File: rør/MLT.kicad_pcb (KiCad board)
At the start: 2 copper layers, 69 x 128.5 mm, 44 parts, among them J1 PJ301M-12, J10 PJ301M-12, J11 PJ301M-12, J12 PJ301M-12, J2 PJ301M-12, J3 PJ301M-12, J4 PJ301M-12, J5 PJ301M-12, J6 PJ301M-12, J7 PJ301M-12, J8 PJ301M-12, J9 PJ301M-12, U1 TL074, U2 TL074, U3 TL074

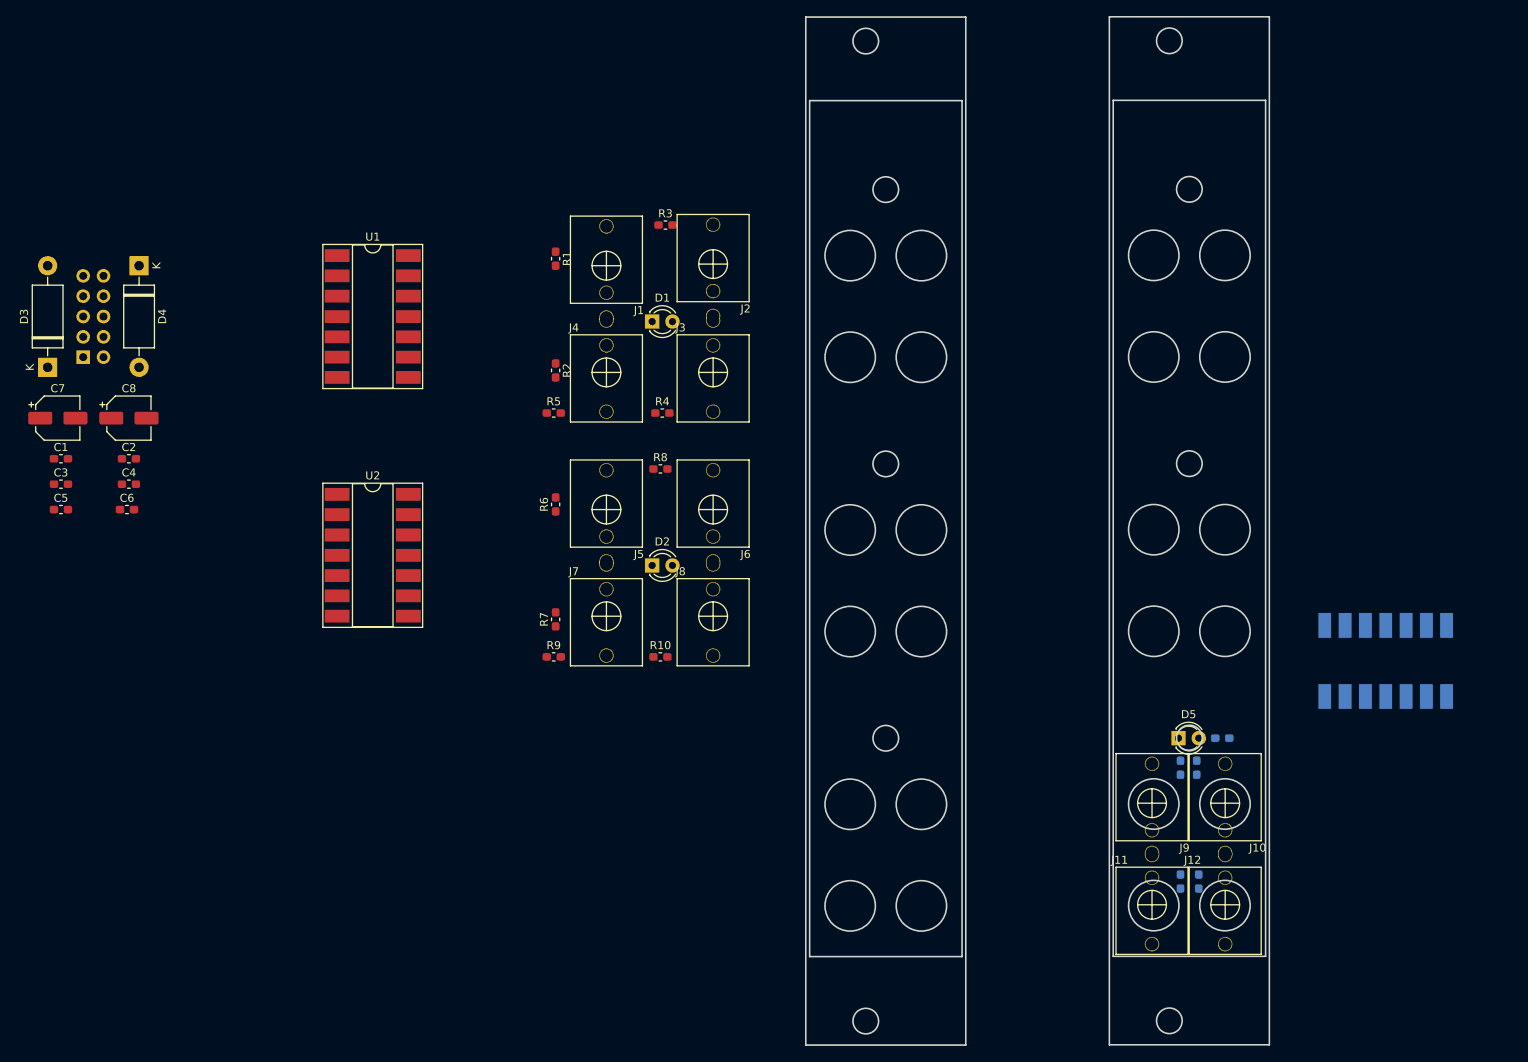
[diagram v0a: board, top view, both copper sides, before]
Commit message: mlt update
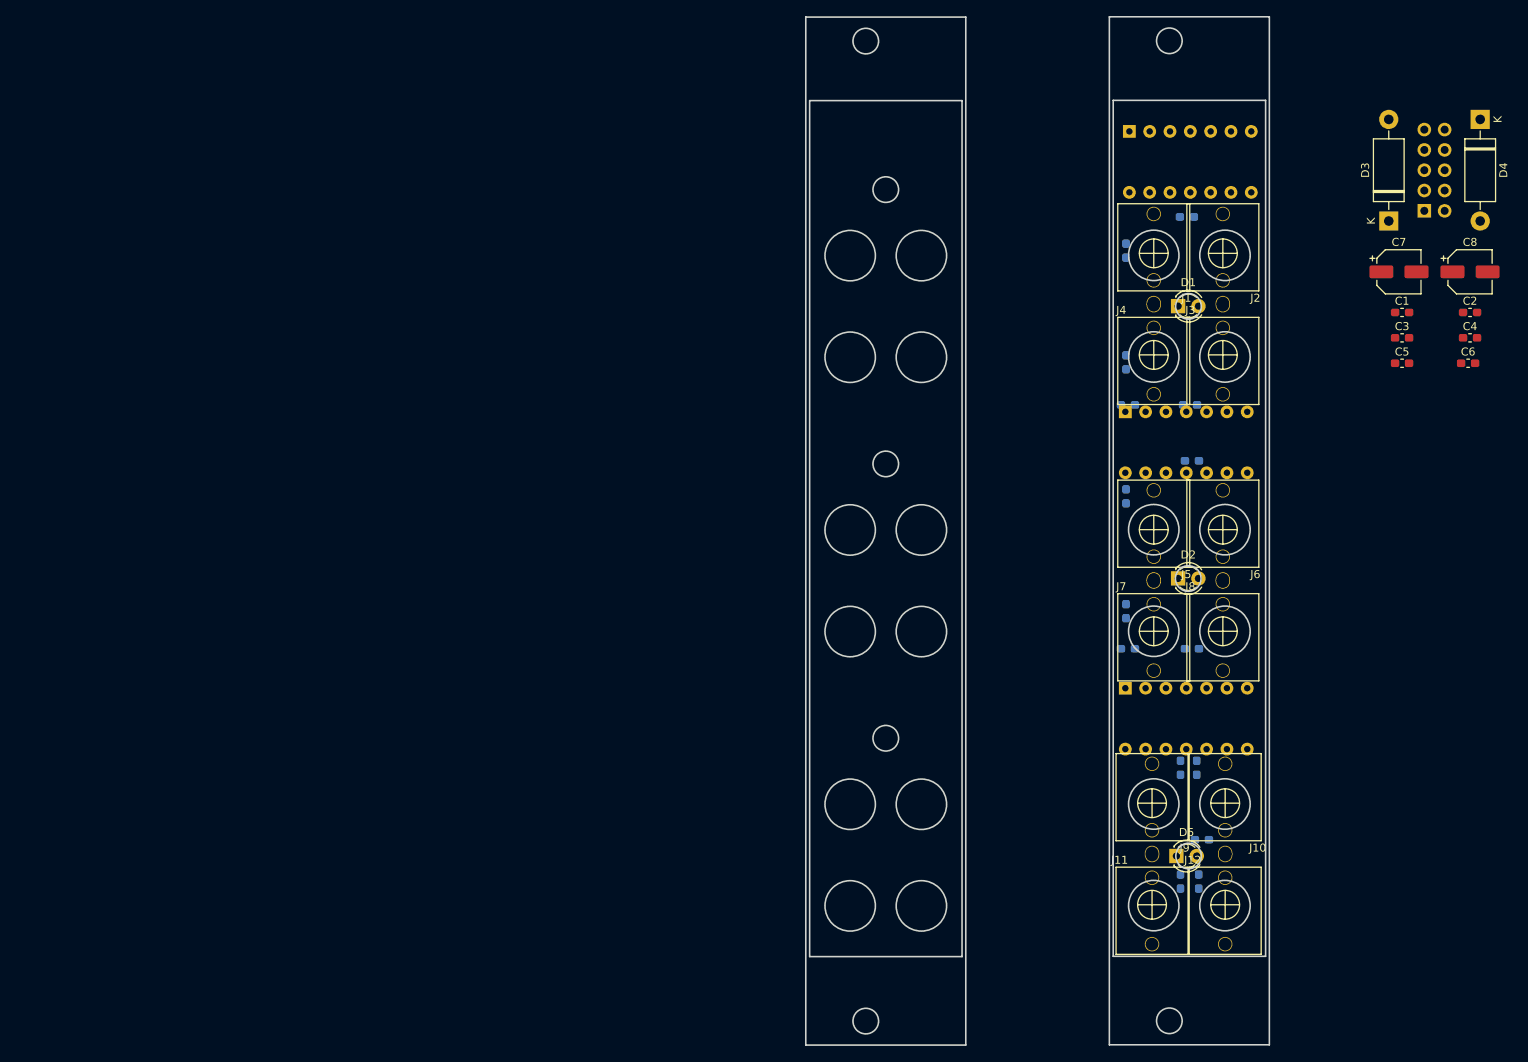
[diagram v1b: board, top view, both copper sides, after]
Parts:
- R1, R10, R2, R3, R4, R5, R6, R7, R8, R9: moved to B.Cu
- U1, U2: footprint Package_DIP:DIP-14_W8.89mm_SMDSocket_LongPads -> Package_DIP:DIP-14_W7.62mm; moved to B.Cu
- U3: footprint Package_DIP:DIP-14_W8.89mm_SMDSocket_LongPads -> Package_DIP:DIP-14_W7.62mm
- moved C2 168.6 mm to (127.6, 68.7)
- moved C4 168.6 mm to (127.6, 71.9)
- moved C7 168.6 mm to (118.7, 63.6)
- moved C8 168.6 mm to (127.6, 63.6)
- moved C1 168.6 mm to (119.1, 68.7)
- moved C3 168.6 mm to (119.1, 71.9)
- moved C5 168.6 mm to (119.1, 75.1)
- moved C6 168.6 mm to (127.4, 75.1)
- moved D3 168.6 mm to (117.5, 57.3)
- moved D4 168.6 mm to (128.9, 44.6)
- moved H1 168.6 mm to (121.9, 56.0)
- moved U1 97.4 mm to (85.1, 46.1), turned to 270 degrees
- moved U2 95.8 mm to (84.5, 81.1), turned to 270 degrees
- moved R5 71.8 mm to (84.9, 80.3), turned to 180 degrees
- moved R9 71.8 mm to (84.9, 110.7), turned to 180 degrees
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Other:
- board size 69 x 128.5 mm -> 57.9 x 128.5 mm
